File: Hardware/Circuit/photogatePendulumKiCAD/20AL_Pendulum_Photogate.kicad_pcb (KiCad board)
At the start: 2 copper layers, 127 x 68.6 mm, 56 parts, among them Q1 2N3906, Q2 2N3904, Q3 2N3904, Q4 BPW40, Q5 2N3904, Q6 2N3904, Q7 2N3904, Q8 2N3904, SW2 SW_SPDT, U2 LM358

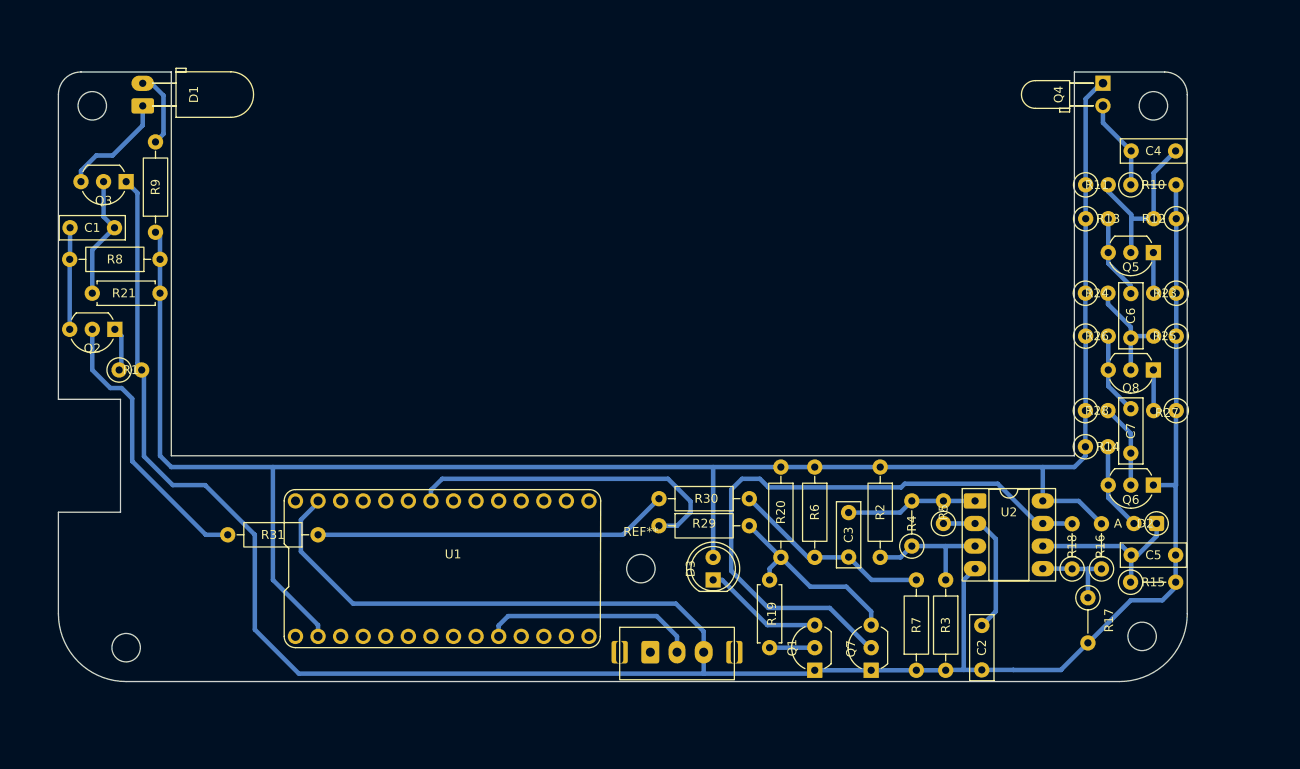
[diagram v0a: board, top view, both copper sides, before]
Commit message: Finalize design
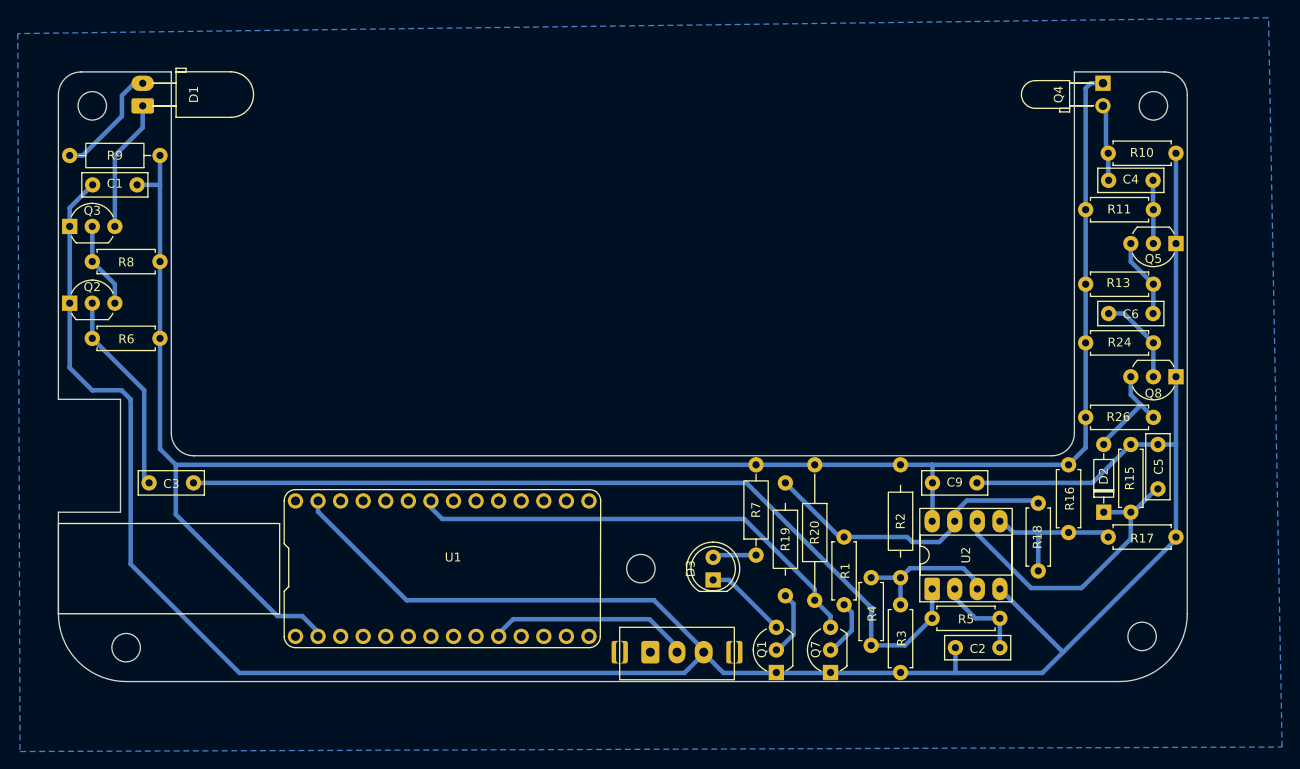
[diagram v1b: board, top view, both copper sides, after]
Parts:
- removed C7: 1n, Capacitor_THT:C_Rect_L7.2mm_W2.5mm_P5.00mm_FKS2_FKP2_MKS2_MKP2
- removed Q6: 2N3904, Package_TO_SOT_THT:TO-92_Inline_Wide
- removed R12, R14: 10k, Resistor_THT:R_Axial_DIN0207_L6.3mm_D2.5mm_P2.54mm_Vertical
- removed R21: 100k, Resistor_THT:R_Axial_DIN0207_L6.3mm_D2.5mm_P7.62mm_Horizontal
- removed R23: 220, Resistor_THT:R_Axial_DIN0207_L6.3mm_D2.5mm_P2.54mm_Vertical
- removed R25: 100k, Resistor_THT:R_Axial_DIN0207_L6.3mm_D2.5mm_P2.54mm_Vertical
- removed R27: 1k, Resistor_THT:R_Axial_DIN0207_L6.3mm_D2.5mm_P2.54mm_Vertical
- removed R28: 1M, Resistor_THT:R_Axial_DIN0207_L6.3mm_D2.5mm_P2.54mm_Vertical
- removed R29, R30, R31: 0, Resistor_THT:R_Axial_DIN0207_L6.3mm_D2.5mm_P10.16mm_Horizontal
- added C9: 10u, Capacitor_THT:C_Rect_L7.2mm_W2.5mm_P5.00mm_FKS2_FKP2_MKS2_MKP2, F.Cu at (123.7, 71.6)
- C1: value 1n -> 10n
- C3: value 10n -> 1n
- C4, C5: value 4n7 -> 1n
- D2: footprint Diode_THT:D_DO-35_SOD27_P2.54mm_Vertical_AnodeUp -> Diode_THT:D_DO-35_SOD27_P7.62mm_Horizontal
- R1: value 2k2 -> 1k; footprint Resistor_THT:R_Axial_DIN0207_L6.3mm_D2.5mm_P2.54mm_Vertical -> Resistor_THT:R_Axial_DIN0207_L6.3mm_D2.5mm_P7.62mm_Horizontal
- R10: value 360 -> 220; footprint Resistor_THT:R_Axial_DIN0207_L6.3mm_D2.5mm_P5.08mm_Vertical -> Resistor_THT:R_Axial_DIN0207_L6.3mm_D2.5mm_P7.62mm_Horizontal
- R11: value 22k -> 100k; footprint Resistor_THT:R_Axial_DIN0207_L6.3mm_D2.5mm_P2.54mm_Vertical -> Resistor_THT:R_Axial_DIN0207_L6.3mm_D2.5mm_P7.62mm_Horizontal
- R13: value 2k2 -> 10k; footprint Resistor_THT:R_Axial_DIN0207_L6.3mm_D2.5mm_P2.54mm_Vertical -> Resistor_THT:R_Axial_DIN0207_L6.3mm_D2.5mm_P7.62mm_Horizontal
- R15, R17, R4: footprint Resistor_THT:R_Axial_DIN0207_L6.3mm_D2.5mm_P5.08mm_Vertical -> Resistor_THT:R_Axial_DIN0207_L6.3mm_D2.5mm_P7.62mm_Horizontal
- R16: value 47k -> 100k; footprint Resistor_THT:R_Axial_DIN0207_L6.3mm_D2.5mm_P5.08mm_Vertical -> Resistor_THT:R_Axial_DIN0207_L6.3mm_D2.5mm_P7.62mm_Horizontal
- R18: value 33k -> 100k; footprint Resistor_THT:R_Axial_DIN0207_L6.3mm_D2.5mm_P5.08mm_Vertical -> Resistor_THT:R_Axial_DIN0207_L6.3mm_D2.5mm_P7.62mm_Horizontal
- R19: value 220 -> 1k; footprint Resistor_THT:R_Axial_DIN0207_L6.3mm_D2.5mm_P7.62mm_Horizontal -> Resistor_THT:R_Axial_DIN0207_L6.3mm_D2.5mm_P10.16mm_Horizontal
- R20: footprint Resistor_THT:R_Axial_DIN0207_L6.3mm_D2.5mm_P10.16mm_Horizontal -> Resistor_THT:R_Axial_DIN0207_L6.3mm_D2.5mm_P15.24mm_Horizontal
- R24: value 220k -> 1M; footprint Resistor_THT:R_Axial_DIN0207_L6.3mm_D2.5mm_P2.54mm_Vertical -> Resistor_THT:R_Axial_DIN0207_L6.3mm_D2.5mm_P7.62mm_Horizontal
- R26: footprint Resistor_THT:R_Axial_DIN0207_L6.3mm_D2.5mm_P2.54mm_Vertical -> Resistor_THT:R_Axial_DIN0207_L6.3mm_D2.5mm_P7.62mm_Horizontal
- R3, R8: footprint Resistor_THT:R_Axial_DIN0207_L6.3mm_D2.5mm_P10.16mm_Horizontal -> Resistor_THT:R_Axial_DIN0207_L6.3mm_D2.5mm_P7.62mm_Horizontal
- R5: value 1k3 -> 1k; footprint Resistor_THT:R_Axial_DIN0207_L6.3mm_D2.5mm_P2.54mm_Vertical -> Resistor_THT:R_Axial_DIN0207_L6.3mm_D2.5mm_P7.62mm_Horizontal
- R6: value 22k -> 1M; footprint Resistor_THT:R_Axial_DIN0207_L6.3mm_D2.5mm_P10.16mm_Horizontal -> Resistor_THT:R_Axial_DIN0207_L6.3mm_D2.5mm_P7.62mm_Horizontal
- R7: value 10k -> 220
- moved R1 83.7 mm to (113.8, 77.7), turned to -90 degrees
- moved R6 75.1 mm to (36.8, 55.4), turned to 180 degrees
- moved C3 73.8 mm to (40.6, 71.6), turned to 180 degrees
- moved R7 22.2 mm to (103.9, 79.8)
- moved C5 12.6 mm to (149.1, 67.3), turned to -90 degrees
- moved R5 12.4 mm to (131.3, 86.9), turned to 180 degrees
- moved U2 11.0 mm to (123.7, 83.6), turned to 90 degrees
- moved R19 9.81 mm to (107.2, 72.9)
- moved R26 9.14 mm to (141.0, 64.3)
- moved R9 8.65 mm to (36.8, 34.8), turned to 180 degrees
- moved Q3 8.11 mm to (26.7, 42.8), turned to 0 degrees
- moved R15 7.87 mm to (146.1, 74.9), turned to 90 degrees
- moved R13 7.37 mm to (141.0, 49.3)
- moved R17 7.20 mm to (143.5, 77.7), turned to 0 degrees
- moved D2 6.07 mm to (143.0, 74.9), turned to 90 degrees
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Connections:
- C1 pad 1: Net-(Q2-C) -> GND
- C1 pad 2: Net-(Q3-B) -> VCC
- C3 pad 2: Net-(C3-Pad2) -> Net-(Q2-B)
- D3 pad 2: VCC -> Net-(D3-A)
- Q2 pad 1: Net-(Q2-E) -> GND
- Q3 pad 2: Net-(Q3-B) -> Net-(Q2-C)
- Q5 pad 1: Net-(Q5-E) -> GND
- Q7 pad 3: Net-(Q7-C) -> INT
- Q8 pad 1: Net-(Q8-E) -> GND
- Q8 pad 3: Net-(Q8-C) -> Net-(D2-A)
- R1 pad 1: Net-(Q2-E) -> Net-(R1-Pad1)
- R1 pad 2: GND -> Net-(Q7-B)
- R18 pad 2: Net-(Q7-B) -> Net-(R1-Pad1)
- R19 pad 1: Net-(Q7-C) -> Net-(R1-Pad1)
- R20 pad 2: Net-(Q7-C) -> INT
- R26 pad 2: Net-(Q8-C) -> Net-(D2-A)
- R6 pad 2: Net-(C3-Pad2) -> Net-(Q2-B)
- R7 pad 1: GND -> Net-(D3-A)
- R7 pad 2: Net-(C3-Pad2) -> VCC
- U2 pad 7: Net-(Q7-B) -> Net-(R1-Pad1)
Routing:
- net Net-(C3-Pad1): track 14.8 -> 97.7 mm
- net Net-(Q7-B): track 69.8 -> 6.54 mm
- net Net-(R30-Pad2): track 40.0 -> 0.00 mm
- net Net-(R1-Pad1): track 0.00 -> 34.2 mm
- net GND: track 288.3 -> 311.6 mm
- net Net-(C3-Pad2): track 22.6 -> 0.00 mm
- net Net-(Q7-C): track 22.3 -> 0.00 mm
- net INT: track 37.4 -> 52.8 mm
- net Net-(D2-K): track 18.6 -> 33.7 mm
- net Net-(Q3-B): track 14.6 -> 0.00 mm
- net Net-(Q5-B): track 19.9 -> 7.13 mm
- net Net-(Q6-B): track 9.45 -> 0.00 mm
- net Net-(Q8-C): track 9.22 -> 0.00 mm
- net Net-(Q2-B): track 31.6 -> 22.9 mm
- net Net-(U2B-+): track 9.90 -> 17.2 mm
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- added copper zone on B.Cu, net GND
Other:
- outline, holes or cut-outs redrawn
- board text removed: "0"
- board text removed: "100k"
- board text removed: "10k"
- board text removed: "10n"
- board text removed: "1M"
- board text removed: "1N4148"
- board text removed: "1k"
- board text removed: "1k3"
- board text removed: "1n"
- board text removed: "220"
- board text removed: "220k"
- board text removed: "22k"
- board text removed: "2N3904"
- board text removed: "2N3906"
- board text removed: "2k2"
- board text removed: "33k"
- board text removed: "360"
- board text removed: "47k"
- board text removed: "4n7"
- board text removed: "Blue LED"
- board text removed: "IR LED"
- board text removed: "LM358"
- board text removed: "Photo"
- board text removed: "SPDT Switch"
- board text removed: "Transistor"
